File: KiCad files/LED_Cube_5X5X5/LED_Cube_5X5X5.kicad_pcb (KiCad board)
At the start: 2 copper layers, 100 x 100 mm, 66 parts, among them J1 Barrel_Jack_MountingPin, J2 USBASP, J3 CON1, J4 CON2, J5 CON3, Q1 BC337, Q2 BC337, Q3 BC337, Q4 BC337, Q5 BC337, SW1 RESET, U1 ATmega16-16PU, U2 74HC595, U3 74HC595, U4 74HC595, U5 74HC595, Y1 16MHz

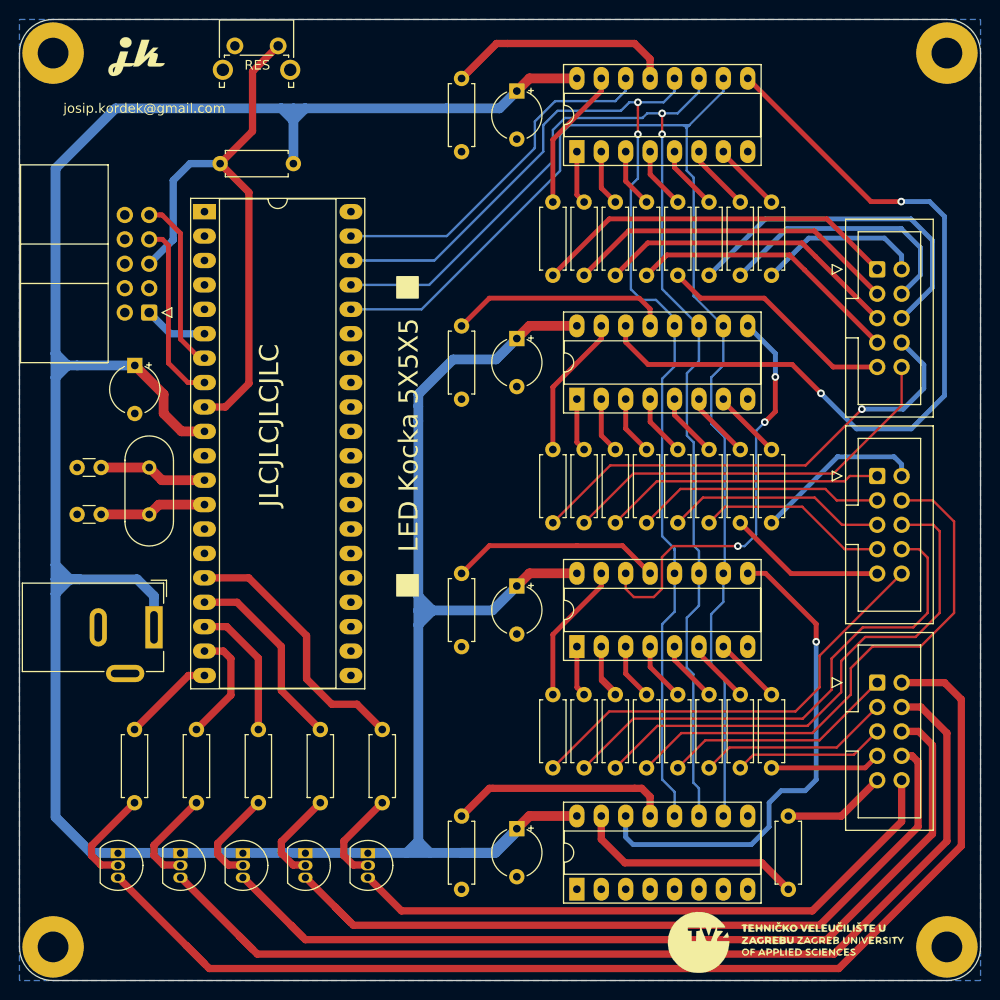
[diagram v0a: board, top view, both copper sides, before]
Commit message: test
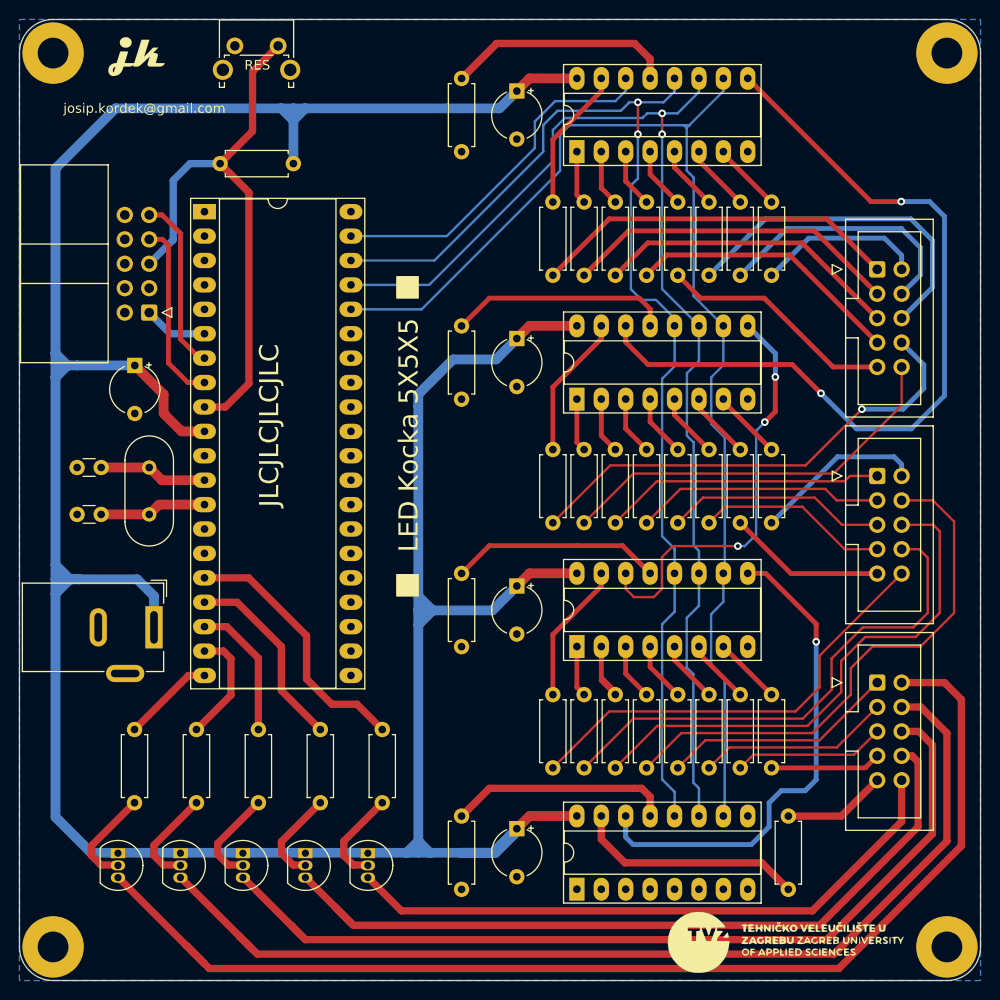
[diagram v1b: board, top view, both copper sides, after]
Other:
- net class Default removed
